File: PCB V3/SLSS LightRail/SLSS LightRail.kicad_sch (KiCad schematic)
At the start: 13 parts, among them J1 Conn_01x04

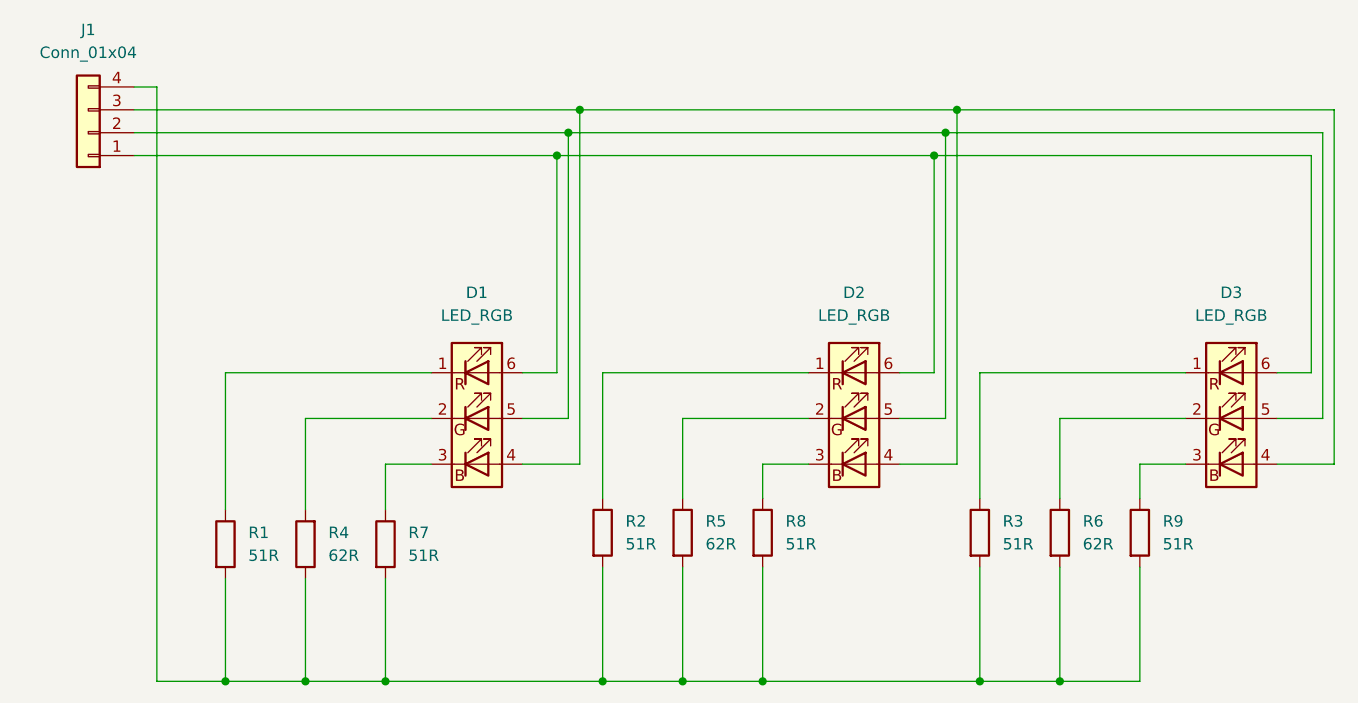
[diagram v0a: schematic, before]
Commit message: Finished Lightrail PCB
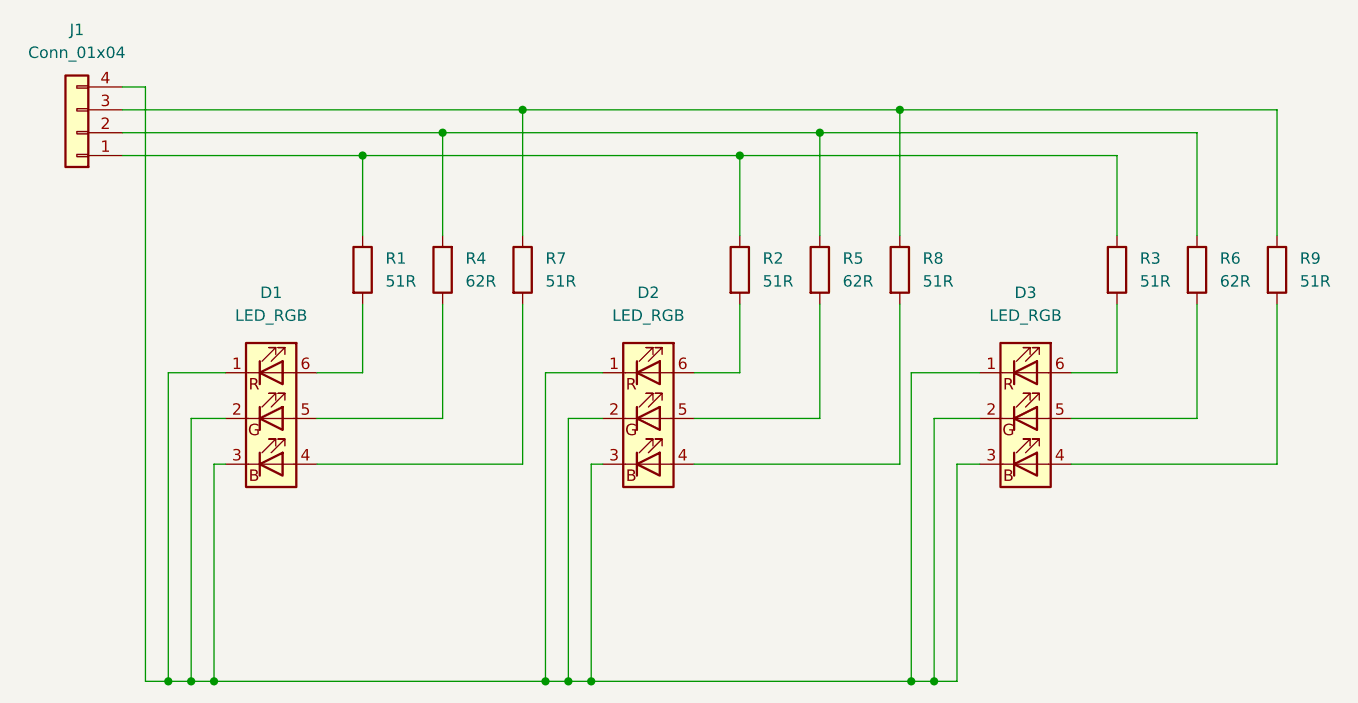
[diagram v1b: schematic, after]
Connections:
- net at R3.1: now also J1.1 (Pin_1), R1.1, R2.1; no longer D3.1 (RK)
- net at D2.1 (RK): now also D1.1 (RK), D1.2 (GK), D1.3 (BK), D2.2 (GK), D2.3 (BK), D3.1 (RK), D3.2 (GK), D3.3 (BK), J1.4 (Pin_4); no longer R2.1
- net at R5.1: now also J1.2 (Pin_2), R4.2, R6.1; no longer D2.2 (GK)
- net at R8.1: now also J1.3 (Pin_3), R7.1, R9.1; no longer D2.3 (BK)
- new net: D3.6 (RA), R3.2
- new net: D2.4 (BA), R8.2
- new net: D2.5 (GA), R5.2
- new net: D2.6 (RA), R2.2
- new net: D3.4 (BA), R9.2
- new net: D1.6 (RA), R1.2
- new net: D1.4 (BA), R7.2
- new net: D1.5 (GA), R4.1
- new net: D3.5 (GA), R6.2
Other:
- moved on the sheet: D1, D2, D3, J1, R1, R2, R3, R4, R5, R6, R7, R8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
